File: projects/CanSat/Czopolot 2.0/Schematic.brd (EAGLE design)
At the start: 45.5 x 30.8 mm, 93 parts

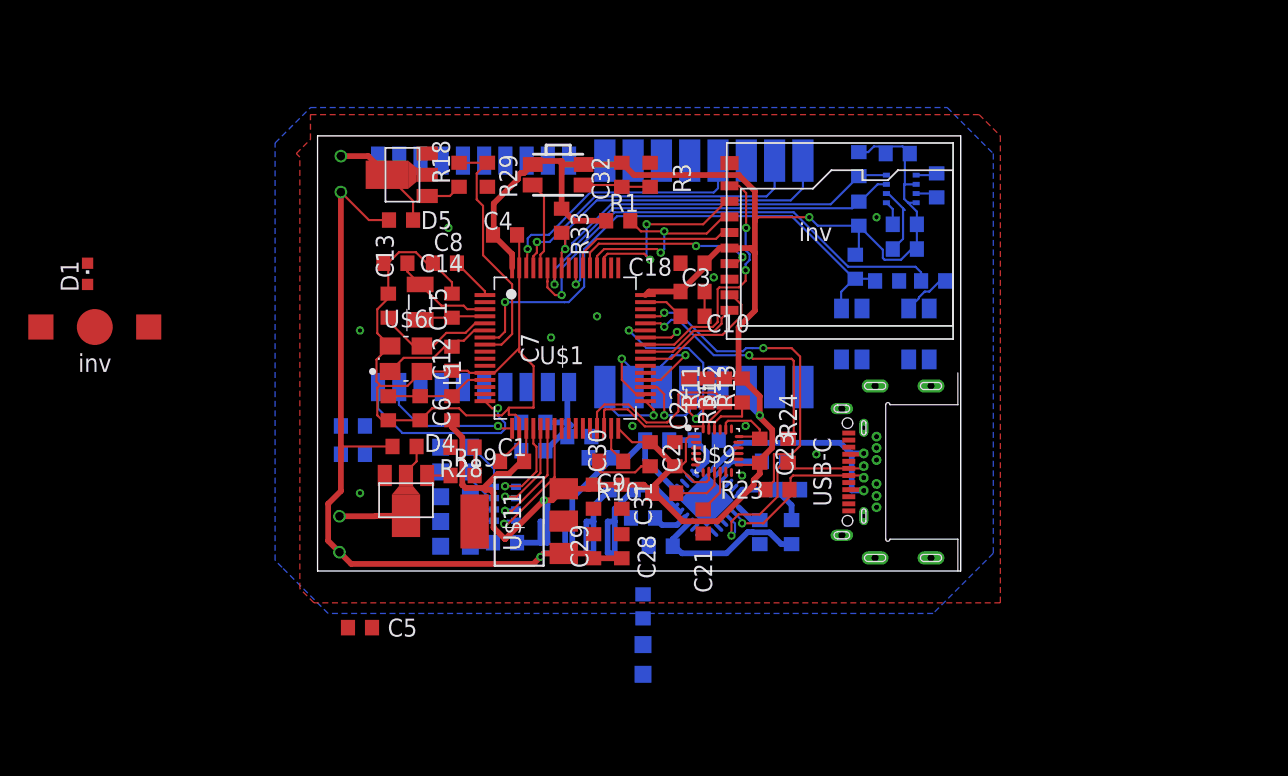
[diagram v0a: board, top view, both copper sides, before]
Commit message: Version 0.2
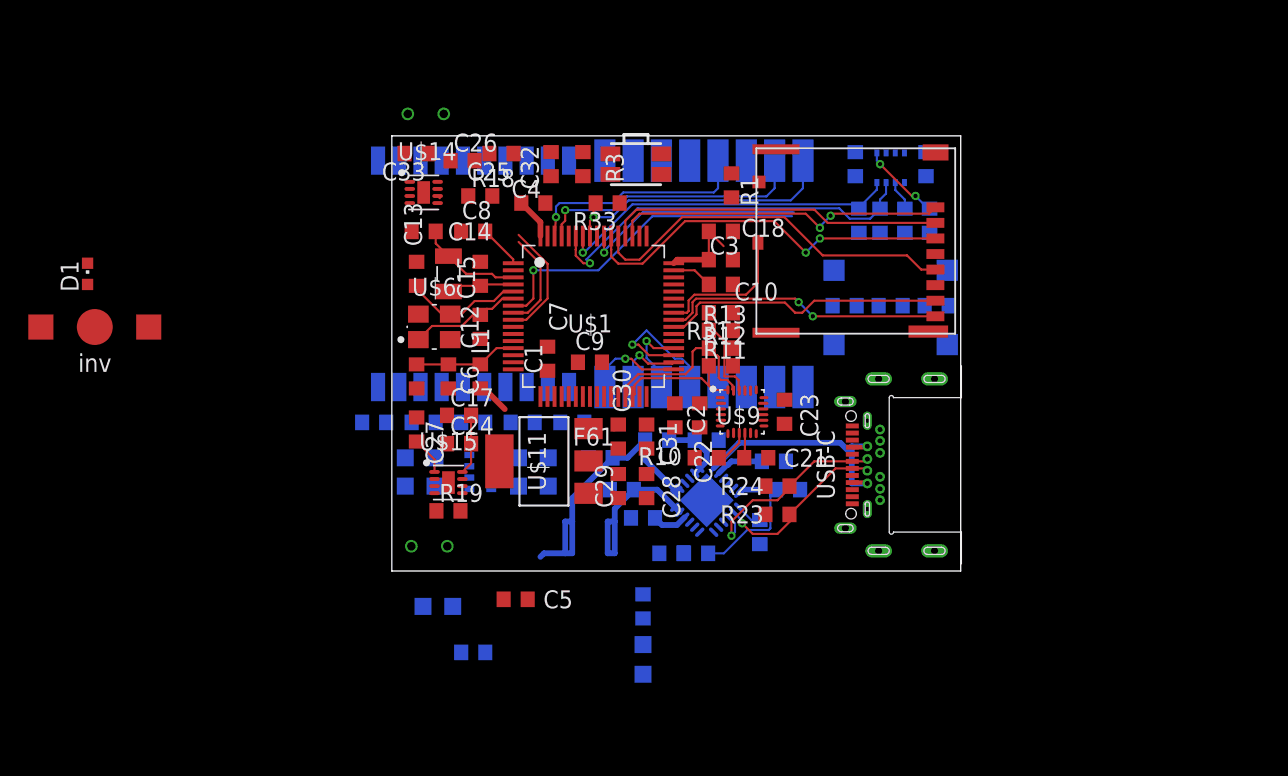
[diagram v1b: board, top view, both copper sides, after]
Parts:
- removed D4, D5: ZENER, Unified:R0603
- removed R28, R29: ?10k, Unified:R0603
- removed U$12, U$13: MOTOR, Unified:INV_MOTOR
- added C17, C25, C27, C33: 100n, Unified:C0603
- added C24, C26: 10u, Unified:C0603
- added MOTL, MOTR: MOTOR, Unified:INV_MOTOR
- BTN_RST, BTN_USR: value PUSH-SWITCH -> PUSH-SWITCHTACT_3X6; device SobieskiSat2:SWITCH_SMD -> SobieskiSat2:TACTHALF_SMD
- R18, R19: value ?10k -> 100k
- U$14, U$15: value NMOSFET -> DRV8838; device SobieskiSat2:INV_SOT-89 -> SobieskiSat2:SON50P200X200X80-9T90X160N
- moved U$15 21.9 mm to (4.50, 6.25), turned to 0 degrees
- moved U$14 20.8 mm to (2.75, 26.8), turned to 0 degrees
- moved C5 11.2 mm to (9.25, -2.00)
- moved R1 8.38 mm to (24.5, 27.2), turned to 270 degrees
- moved R30 8.07 mm to (6.25, -5.75)
- moved C1 7.67 mm to (11.5, 15.0), turned to 270 degrees
- moved C9 7.16 mm to (14.5, 14.8), turned to 0 degrees
- moved R16 6.91 mm to (22.0, 1.25), turned to 180 degrees
- moved R4 6.49 mm to (32.5, 18.8)
- moved R2 6.37 mm to (39.0, 18.8), turned to 180 degrees
- moved D6 6.04 mm to (10.5, 6.00), turned to 90 degrees
- moved R31 5.94 mm to (23.8, 18.2), turned to 180 degrees
- moved C21 5.86 mm to (26.2, 8.00), turned to 180 degrees
- moved BTN_DFU 5.55 mm to (17.8, 28.8)
- moved D9 5.55 mm to (10.5, 8.00), turned to 90 degrees
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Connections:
- removed net IN_MOT1: R19.2, R28.2
- removed net IN_MOT2: R18.2, R29.2, U$1.8
- removed net N$4 (its old number): U$1.42
- removed net N$41: D5.1, U$13.P$1, U$15.2, U$15.2@1
- removed net N$42: D4.1, U$12.P$1, U$14.2, U$14.2@1
- removed net N$43: D6.A, RN1.1
- removed net N$44: D7.A, RN1.2
- removed net N$45: D8.A, RN1.3
- removed net N$49: D9.A, RN1.4
- removed net N$50: RN1.5, U$1.20
- new net DAC1: U$1.20
- new net DAC2: U$1.21
- new net EN_L: U$1.8, U$14.5
- new net EN_R: U$1.15, U$15.5
- new net N$29: RN1.3, U$1.23
- new net N$30: C25.2, C26.2, U$14.8
- new net N$31: R18.1, U$14.7
- new net N$32: RN1.2, U$1.24
- new net N$33: RN1.1, U$1.25
- new net N$34: MOTR.P$2, U$15.2
- new net N$36: MOTR.P$1, U$15.3
- new net N$37: D7.A, RN1.7
- new net N$38: D6.A, RN1.8
- new net N$39: C17.2, C24.2, U$15.8
- new net N$40: R19.1, U$15.7
- new net PH_L: U$1.9, U$14.6
- new net PH_R: U$1.14, U$15.6
- net GND: now also C17.1, C24.1, C25.1, C26.1, C27.1, C33.1, U$14.4, U$14.9, U$15.4, U$15.9, U$2.GND, U$2.SW2; no longer BTN_RST.P$4, BTN_USR.P$4, R28.1, R29.1, U$14.3, U$15.3, U$2.P$10, U$2.P$6
- net N$1: now also D9.A, RN1.5; no longer RN1.8, U$1.23
- net N$16: no longer BTN_USR.P$3
- net N$2: now also D8.A; no longer U$1.21
- net N$26: now also MOTL.P$1, U$14.3; no longer R19.1, U$14.1
- net N$3: now also RN1.4; no longer RN1.7
- net N$5: now also MOTL.P$2, U$14.2; no longer R18.1, U$15.1
- net N$7: no longer BTN_RST.P$3
- net SD_CLK: now also U$2.CLK; no longer U$2.P$5
- net SD_CMD: now also U$2.CMD; no longer U$2.P$3
- net SD_D0: now also U$2.D0; no longer U$2.P$7
- net SD_D1: now also U$2.D1; no longer U$2.P$8
- net SD_D2: now also U$2.D2; no longer U$2.P$1
- net SD_D3: now also U$2.D3; no longer U$2.P$2
- net SD_SW: now also U$2.SW1; no longer U$2.P$9
- net VCC: now also R18.2, R19.2, U$2.VCC; no longer U$2.P$4
- net VSYS: now also C27.2, C33.2, U$14.1, U$15.1; no longer D4.2, D5.2, U$12.P$2, U$13.P$2
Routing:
- net VCC: track 161.7 -> 13.8 mm, vias 3 -> 0
- net GND: track 82.8 -> 0.00 mm, vias 11 -> 0
- net VSYS: track 75.7 -> 24.1 mm, vias 1 -> 0
- net N$35: track 23.7 -> 0.00 mm, vias 2 -> 0
- net IN_MOT2: track 17.7 -> 0.00 mm
- net N$25: track 17.4 -> 0.00 mm, vias 2 -> 0
- net N$15: track 31.4 -> 15.9 mm
- net SD_CMD: track 12.0 -> 27.1 mm, vias 0 -> 2
- net N$7: track 38.3 -> 23.5 mm
- net GPS_RX: track 14.1 -> 0.00 mm, vias 1 -> 0
- net SD_CLK: track 13.6 -> 26.6 mm, vias 2 -> 0
- net N$4: track 12.9 -> 0.00 mm, vias 2 -> 0
- net SD_D1: track 7.38 -> 20.1 mm, vias 0 -> 2
- net N$22: track 11.8 -> 0.00 mm
- net N$10: track 11.3 -> 0.00 mm
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- removed copper zone on layer 1, net GND
- removed copper zone on layer 16, net GND
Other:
- board size 45.5 x 30.8 mm -> 40.2 x 30.8 mm
- board text added: "^ Battery and switch holes or pads"

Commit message: Version 0.3
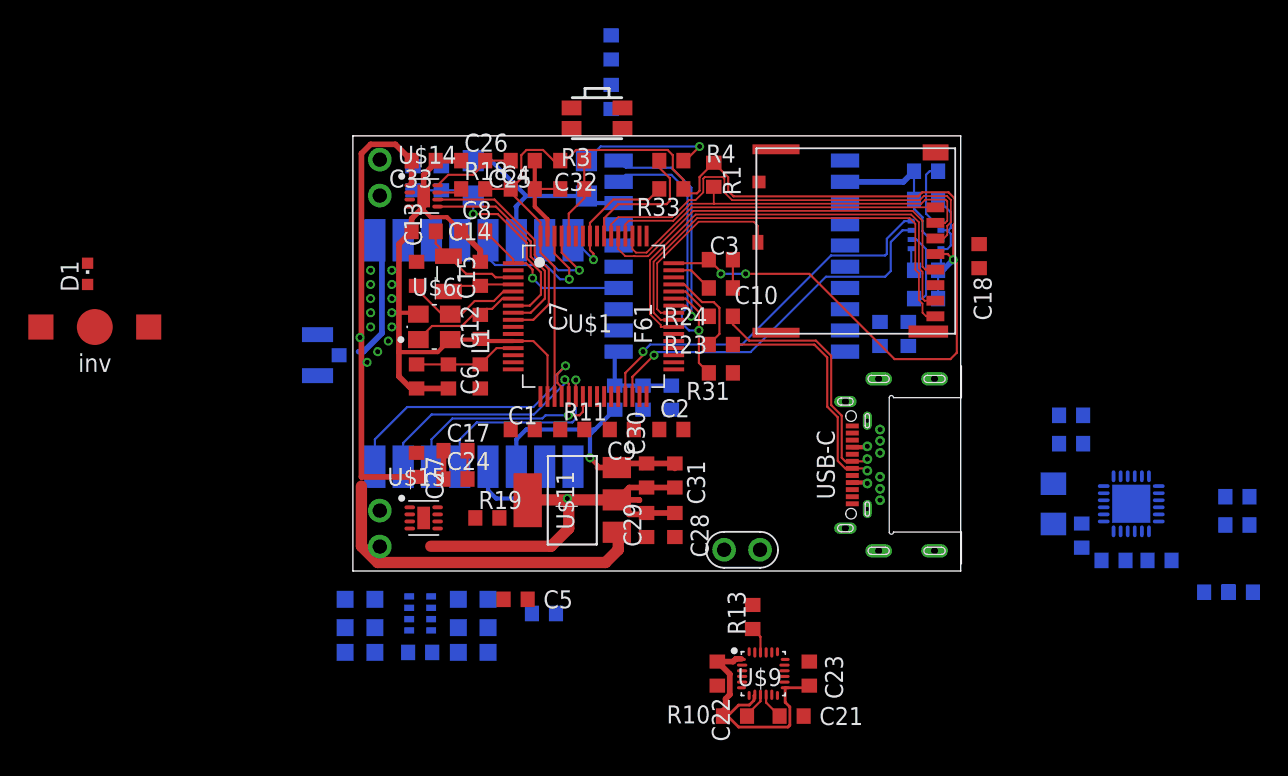
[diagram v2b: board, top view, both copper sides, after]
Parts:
- removed R12: 10k, Unified:R0603
- added BAT_PACK: (no value), SobieskiSat2:2X1_2.54
- added U$12: 50R, SobieskiSat2:CON_U.FL
- L2: device Unified:R0603 -> Unified:R1206
- MOTL, MOTR: device Unified:INV_MOTOR -> Unified:2X1_2.54
- R11: value 10k -> 100k
- moved R16 38.6 mm to (60.5, -1.50)
- moved R17 38.6 mm to (58.8, -1.50)
- moved R15 36.6 mm to (54.8, 0.75), turned to 0 degrees
- moved R2 36.1 mm to (4.00, 27.8), turned to 90 degrees
- moved C16 35.1 mm to (51.5, 0.75)
- moved C11 34.9 mm to (2.00, 27.8), turned to 270 degrees
- moved C35 34.4 mm to (49.2, 2.50), turned to 270 degrees
- moved R14 33.8 mm to (60.2, 5.25), turned to 180 degrees
- moved C37 31.8 mm to (60.2, 3.25), turned to 180 degrees
- moved D61 31.3 mm to (16.0, 37.0), turned to 90 degrees
- moved U$10 30.0 mm to (52.8, 4.75), turned to 0 degrees
- moved L2 28.4 mm to (47.2, 4.75), turned to 90 degrees
- moved BTN_RST 27.6 mm to (10.2, 26.5)
- moved BTN_USR 26.7 mm to (10.2, 29.0), turned to 180 degrees
- moved R63 26.5 mm to (16.0, 33.5), turned to 90 degrees
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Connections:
- net N$10 renamed DFU
- net N$7 renamed NRST
- removed net BMP_SCL: R6.1, U$1.58, U$8.4
- removed net BMP_SDA: R7.1, U$1.59, U$8.3
- removed net DAC1: U$1.20
- removed net DAC2: U$1.21
- removed net MPU_SCL: R12.1, U$1.29, U$9.23
- removed net MPU_SDA: R11.1, U$1.30, U$9.24
- removed net N$19: B6.P$1, U$3.P$4
- removed net N$29: RN1.3, U$1.23
- removed net N$3: RN1.4, U$1.22
- removed net N$32: RN1.2, U$1.24
- removed net N$33: RN1.1, U$1.25
- removed net N$4 (its old number): R31.2, U$1.43
- new net N$7: R11.2, U$1.28
- new net SCL: R7.2, U$1.29, U$8.4, U$9.23
- new net SDA: R6.2, U$1.30, U$8.3, U$9.24
- net BAT: now also BAT_PACK.P$1
- net GND: now also BAT_PACK.P$2, R11.1, U$12.GND, U$12.GND@1
- net GPS_RX: now also U$1.42; no longer U$1.16
- net GPS_TX: now also R31.2, U$1.43; no longer U$1.17
- net LR_ANT: now also U$12.SIG
- net LR_MISO: now also U$1.22; no longer U$1.35
- net LR_MOSI: now also U$1.23; no longer U$1.36
- net LR_NSS: now also U$1.20; no longer U$1.33
- net LR_SCK: now also U$1.21; no longer U$1.34
- net VBACKUP: now also B6.P$1, U$3.P$4
- net VCC: now also R6.1, R7.1; no longer R11.2, R12.2, R6.2, R7.2
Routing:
- net VCC: track 13.8 -> 142.5 mm, vias 0 -> 4
- net GND: track 0.00 -> 122.1 mm, vias 0 -> 15
- net VSYS: track 24.1 -> 57.4 mm
- net BMP_SDA: track 27.9 -> 0.00 mm, vias 1 -> 0
- net SCL: track 0.00 -> 27.1 mm, vias 0 -> 1
- net SDA: track 0.00 -> 26.6 mm, vias 0 -> 1
- net BMP_SCL: track 24.6 -> 0.00 mm, vias 1 -> 0
- net GPS_TX: track 0.00 -> 23.2 mm, vias 0 -> 1
- net GPS_RX: track 0.00 -> 16.8 mm, vias 0 -> 1
- net USB_VBUS: track 17.8 -> 2.17 mm
- net LR_NSS: track 6.74 -> 20.5 mm
- net SD_D0: track 20.2 -> 33.0 mm
- net SD_D1: track 20.1 -> 32.7 mm, vias 2 -> 0
- net MPU_SCL: track 12.4 -> 0.00 mm
- net LR_BUSY: track 19.3 -> 6.95 mm
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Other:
- board size 40.2 x 30.8 mm -> 43 x 30.8 mm
